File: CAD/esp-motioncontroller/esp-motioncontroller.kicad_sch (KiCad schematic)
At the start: 4 parts

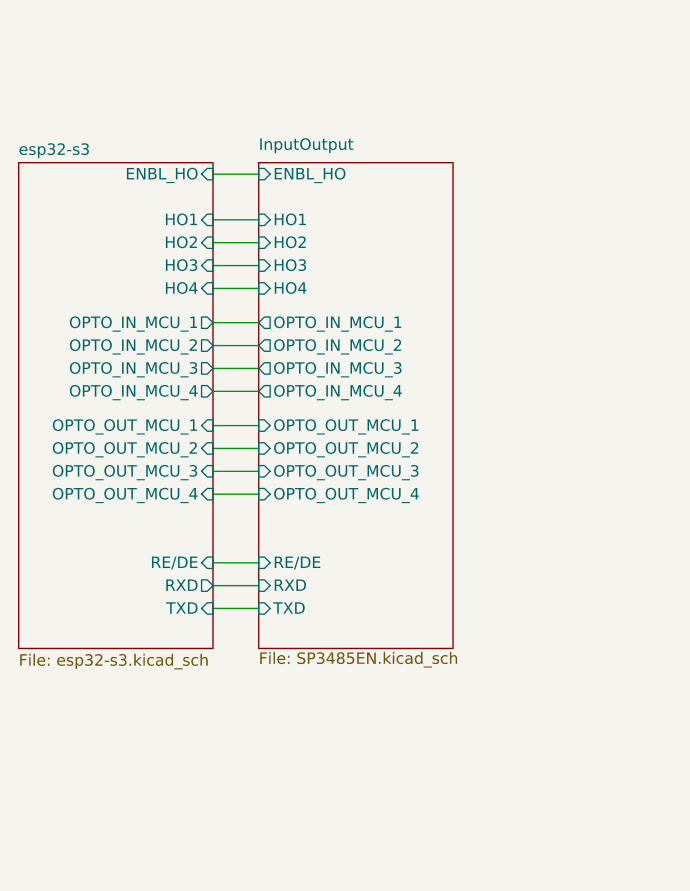
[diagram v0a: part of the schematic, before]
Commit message: Feat: Quaddrivers
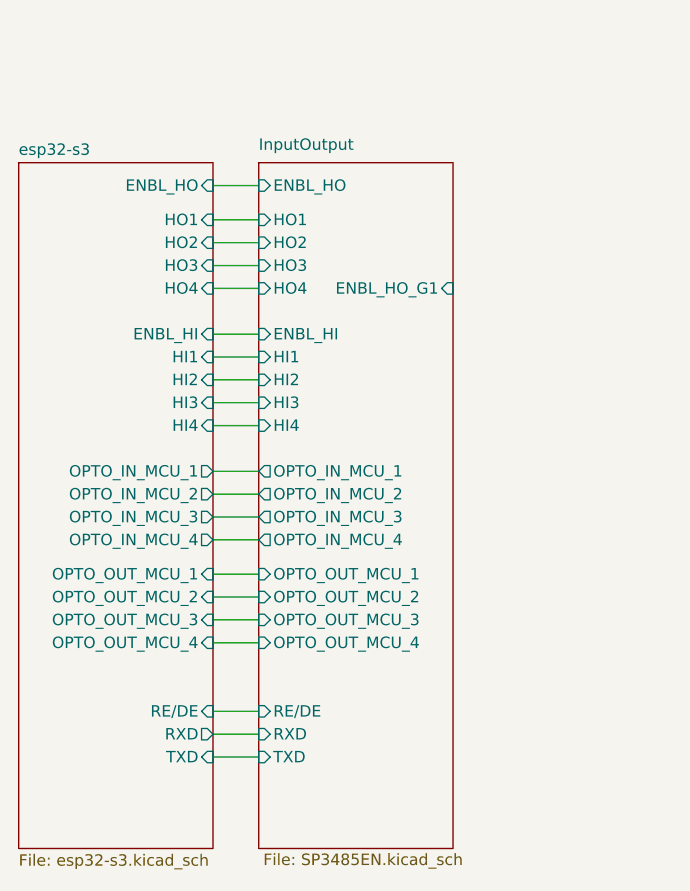
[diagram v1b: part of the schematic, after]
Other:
- sheet InputOutput ports: added ENBL_HI, ENBL_HO_G1, HI1, HI2, HI3, HI4; removed none
- sheet esp32-s3 ports: added ENBL_HI, HI1, HI2, HI3, HI4; removed none
